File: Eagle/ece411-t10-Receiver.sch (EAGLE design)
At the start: 10 parts, among them X1 22-23-2021, X2 22-23-2021

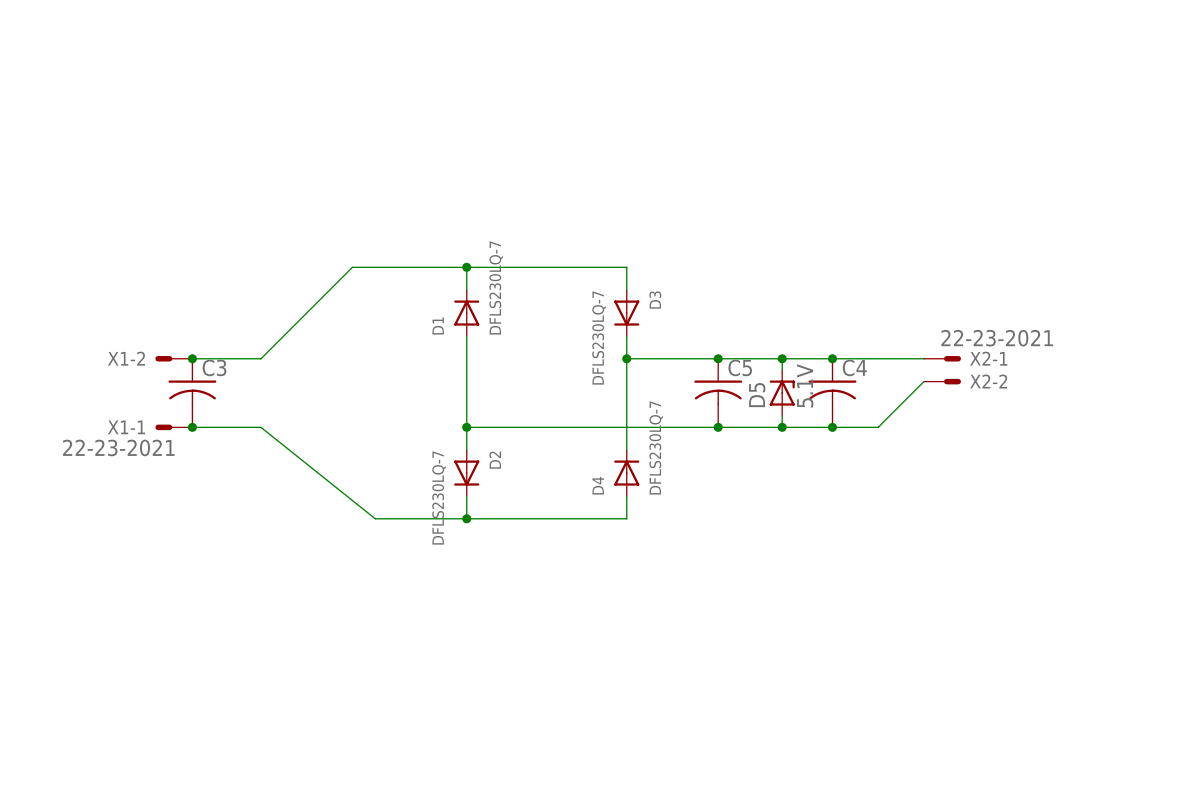
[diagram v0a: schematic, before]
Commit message: Boards + schematics rev2
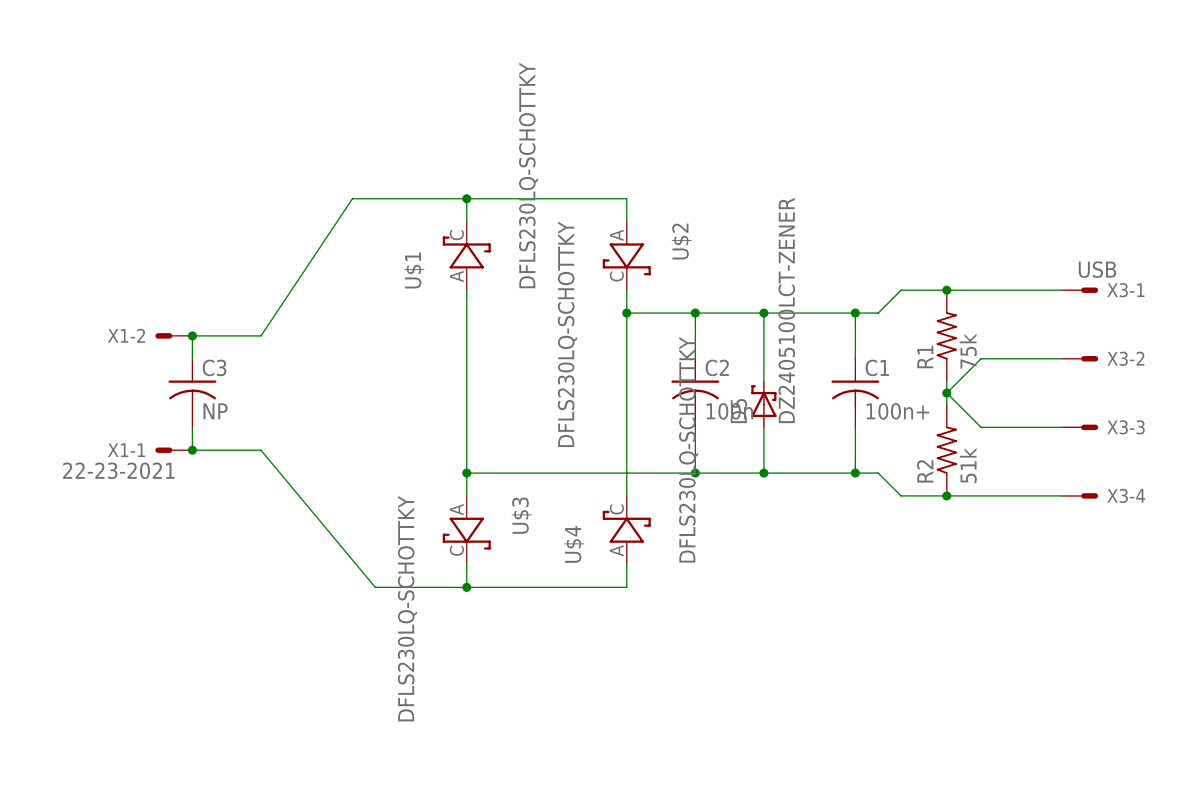
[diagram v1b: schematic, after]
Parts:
- removed C4, C5: (no value), adafruit:C-USC0805
- removed D1, D2, D3, D4: DFLS230LQ-7, adafruit:DIODESOD-523
- removed X2: 22-23-2021, con-molex:22-23-2021
- added C1: 100n+, adafruit:C-USC0805
- added C2: 100n, adafruit:C-USC0805
- added R1: 75k, resistor:R-US_R0805
- added R2: 51k, resistor:R-US_R0805
- added U$1, U$2, U$3, U$4: DFLS230LQ-SCHOTTKY, _VMS:DFLS230LQ-SCHOTTKY
- added X3: USB, con-molex:22-23-2041
- C3: value (none) -> NP
- D5: value 5.1V -> DZ2405100LCT-ZENER; device diode:BZX84CSMD -> _VMS:DZ2405100LCT-ZENER
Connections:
- removed net N$3: C4.2, C5.2, D1.A, D2.A, D5.A, X2-2.S
- new net N$5: R1.1, R2.2, X3-2.S, X3-3.S
- new net N$8: C1.2, C2.2, D5.A, R2.1, U$1.A, U$3.A, X3-4.S
- net N$1: now also U$1.C, U$2.A; no longer D1.C, D3.A
- net N$2: now also U$3.C, U$4.A; no longer D2.C, D4.A
- net N$4: now also C1.1, C2.1, R1.2, U$2.C, U$4.C, X3-1.S; no longer C4.1, C5.1, D3.C, D4.C, X2-1.S
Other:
- moved on the sheet: X1-1, X1-2
